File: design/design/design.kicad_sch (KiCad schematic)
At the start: 29 parts, among them J1 Impulse, J2 Voltage, J3 OUT, U1 TL084CN, U2 TL084CN, U3 TL084CN

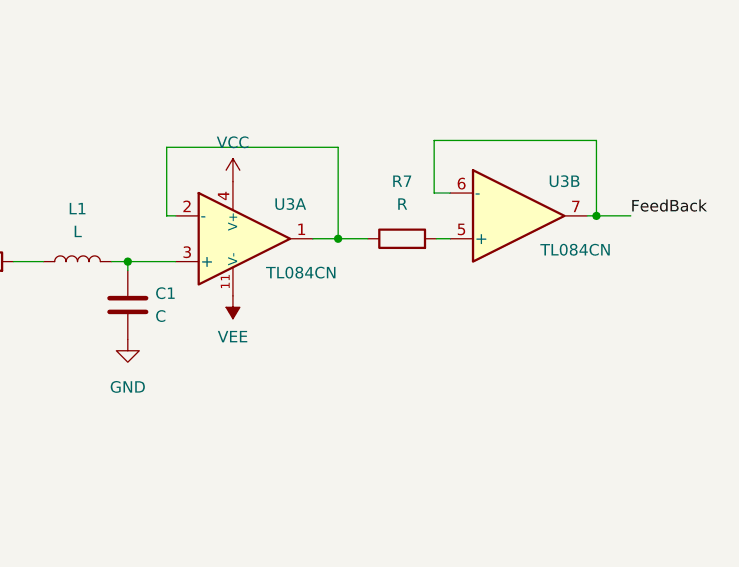
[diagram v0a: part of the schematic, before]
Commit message: fix: add cap on pcb and design
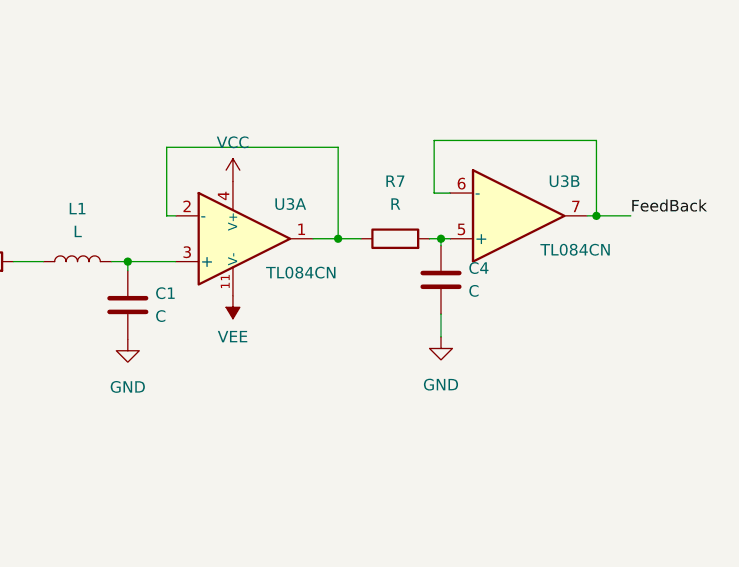
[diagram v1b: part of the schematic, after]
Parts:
- added C4: C, Capacitor_THT:C_Disc_D5.0mm_W2.5mm_P5.00mm, symbol Device:C
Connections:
- net GND: now also C4.1
- net at R7.2, U3.5 (+): now also C4.2
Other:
- moved on the sheet: R7
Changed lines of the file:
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@@
 	)
 	(junction
+		(at 256.286 64.008)
+		(diameter 0)
+		(color 0 0 0 0)
+	)
+	(junction
 		(at 122.428 28.194)
 		(diameter 0)
@@
 	(wire
 		(pts
+			(xy 256.286 64.77) (xy 256.286 64.008)
+		)
+		(stroke
+			(width 0)
+			(type default)
+		)
+	)
+	(wire
+		(pts
 			(xy 208.788 66.548) (xy 212.09 66.548)
 		)
@@
 	(wire
 		(pts
+			(xy 256.286 74.93) (xy 256.286 72.39)
+		)
+		(stroke
+			(width 0)
+			(type default)
+		)
+	)
+	(wire
+		(pts
 			(xy 146.558 30.734) (xy 146.558 63.754)
 		)
@@
 	(wire
 		(pts
+			(xy 256.286 64.008) (xy 257.302 64.008)
+		)
+		(stroke
+			(width 0)
+			(type default)
+		)
+	)
+	(wire
+		(pts
 			(xy 70.358 47.244) (xy 70.358 61.214)
 		)
@@
 	(wire
 		(pts
-			(xy 255.778 64.008) (xy 257.302 64.008)
+			(xy 255.016 64.008) (xy 256.286 64.008)
 		)
 		(stroke
@@
 	(wire
 		(pts
-			(xy 242.062 64.008) (xy 248.158 64.008)
+			(xy 242.062 64.008) (xy 247.396 64.008)
 		)
 		(stroke
@@
 	)
 	(symbol
+		(lib_id "Device:C")
+		(at 256.286 68.58 180)
+		(unit 1)
+		(body_style 1)
+		(exclude_from_sim no)
+		(in_bom yes)
+		(on_board yes)
+		(in_pos_files yes)
+		(dnp no)
+		(fields_autoplaced yes)
+		(property "Reference" "C4"
+			(at 259.334 67.3099 0)
+			(show_name no)
+			(do_not_autoplace no)
+			(effects
+				(font
+					(size 1.27 1.27)
+				)
+				(justify right)
+			)
+		)
+		(property "Value" "C"
+			(at 259.334 69.8499 0)
+			(show_name no)
+			(do_not_autoplace no)
+			(effects
+				(font
+					(size 1.27 1.27)
+				)
+				(justify right)
+			)
+		)
+		(property "Footprint" "Capacitor_THT:C_Disc_D5.0mm_W2.5mm_P5.00mm"
+			(at 255.3208 64.77 0)
+			(hide yes)
+			(show_name no)
+			(do_not_autoplace no)
+			(effects
+				(font
+					(size 1.27 1.27)
+				)
+			)
+		)
+		(property "Datasheet" ""
+			(at 256.286 68.58 0)
+			(hide yes)
+			(show_name no)
+			(do_not_autoplace no)
+			(effects
+				(font
+					(size 1.27 1.27)
+				)
+			)
+		)
+		(property "Description" "Unpolarized capacitor"
+			(at 256.286 68.58 0)
+			(hide yes)
+			(show_name no)
+			(do_not_autoplace no)
+			(effects
+				(font
+					(size 1.27 1.27)
+				)
+			)
+		)
+		(pin "2"
+		)
+		(pin "1"
+		)
+		(instances
+			(project "design"
+				(path "/bb8eacac-7b7c-407c-b2e2-d96fde64f67b"
+					(reference "C4")
+					(unit 1)
+				)
+			)
+		)
+	)
+	(symbol
 		(lib_id "power:VCC")
 		(at 110.998 20.574 0)
@@
 	)
 	(symbol
+		(lib_id "power:GND")
+		(at 256.286 74.93 0)
+		(mirror y)
+		(unit 1)
+		(body_style 1)
+		(exclude_from_sim no)
+		(in_bom yes)
+		(on_board yes)
+		(in_pos_files yes)
+		(dnp no)
+		(property "Reference" "#PWR013"
+			(at 256.286 81.28 0)
+			(hide yes)
+			(show_name no)
+			(do_not_autoplace no)
+			(effects
+				(font
+					(size 1.27 1.27)
+				)
+			)
+		)
+		(property "Value" "GND"
+			(at 256.286 80.264 0)
+			(show_name no)
+			(do_not_autoplace no)
+			(effects
+				(font
+					(size 1.27 1.27)
+				)
+			)
+		)
+		(property "Footprint" ""
+			(at 256.286 74.93 0)
+			(hide yes)
+			(show_name no)
+			(do_not_autoplace no)
+			(effects
+				(font
+					(size 1.27 1.27)
+				)
+			)
+		)
+		(property "Datasheet" ""
+			(at 256.286 74.93 0)
+			(hide yes)
+			(show_name no)
+			(do_not_autoplace no)
+			(effects
+				(font
+					(size 1.27 1.27)
+				)
+			)
+		)
+		(property "Description" "Power symbol creates a global label with name \"GND\" , ground"
+			(at 256.286 74.93 0)
+			(hide yes)
+			(show_name no)
+			(do_not_autoplace no)
+			(effects
+				(font
+					(size 1.27 1.27)
+				)
+			)
+		)
+		(pin "1"
+		)
+		(instances
+			(project "design"
+				(path "/bb8eacac-7b7c-407c-b2e2-d96fde64f67b"
+					(reference "#PWR013")
+					(unit 1)
+				)
+			)
+		)
+	)
+	(symbol
 		(lib_id "PCM_SL_Pin_Headers:PINHD_1x2_Male")
 		(at 192.024 118.872 0)
@@
 	(symbol
 		(lib_id "Device:R")
-		(at 251.968 64.008 90)
+		(at 251.206 64.008 90)
 		(unit 1)
 		(body_style 1)
@@
 		(fields_autoplaced yes)
 		(property "Reference" "R7"
-			(at 251.968 57.658 90)
+			(at 251.206 57.658 90)
 			(show_name no)
 			(do_not_autoplace no)
@@
 		)
 		(property "Value" "R"
-			(at 251.968 60.198 90)
+			(at 251.206 60.198 90)
 			(show_name no)
 			(do_not_autoplace no)
@@
 		)
 		(property "Footprint" "Resistor_THT:R_Axial_DIN0207_L6.3mm_D2.5mm_P10.16mm_Horizontal"
-			(at 251.968 65.786 90)
+			(at 251.206 65.786 90)
 			(hide yes)
 			(show_name no)
@@
 		)
 		(property "Datasheet" ""
-			(at 251.968 64.008 0)
+			(at 251.206 64.008 0)
 			(hide yes)
 			(show_name no)
@@
 		)
 		(property "Description" "Resistor"
-			(at 251.968 64.008 0)
+			(at 251.206 64.008 0)
 			(hide yes)
 			(show_name no)
